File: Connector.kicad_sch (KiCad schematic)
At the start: 1 part, among them J6 2-338069-0

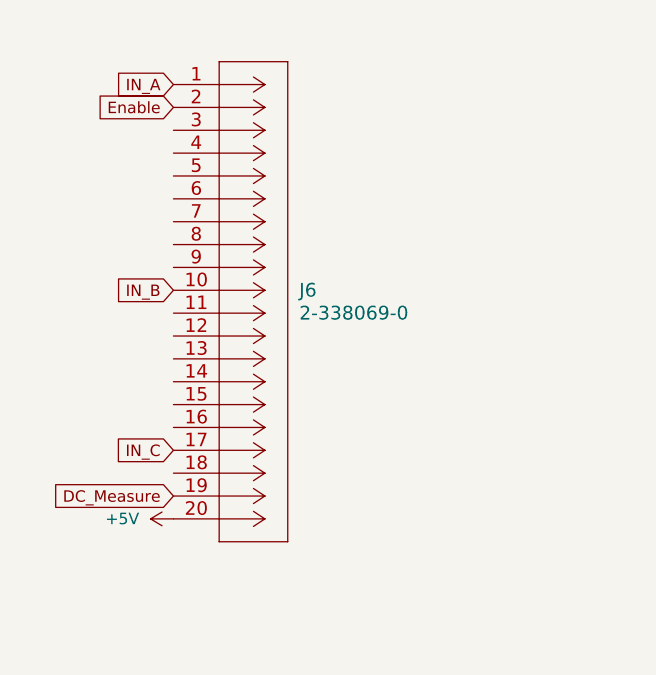
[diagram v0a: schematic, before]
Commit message: Стартовый вариант
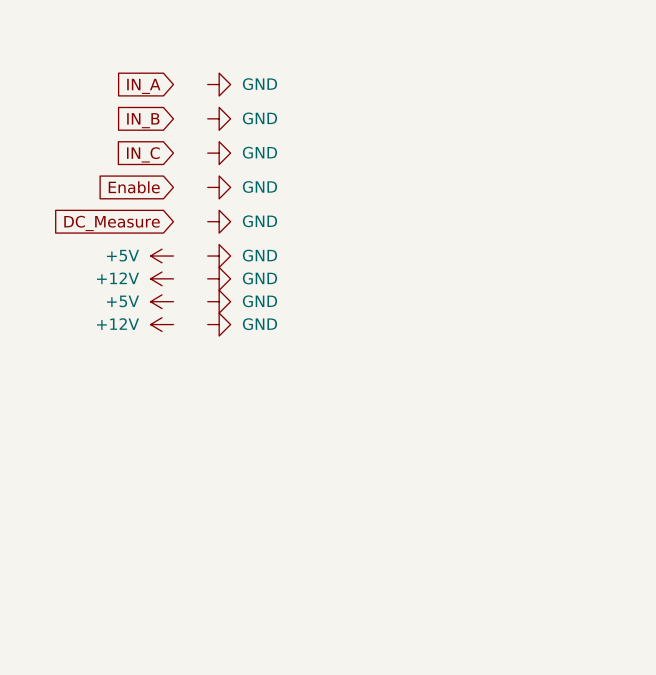
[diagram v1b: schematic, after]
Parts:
- removed J6: 2-338069-0, Connector_My:2-338069-0, symbol Connector_My:2-338069-0

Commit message: Стартовая версия
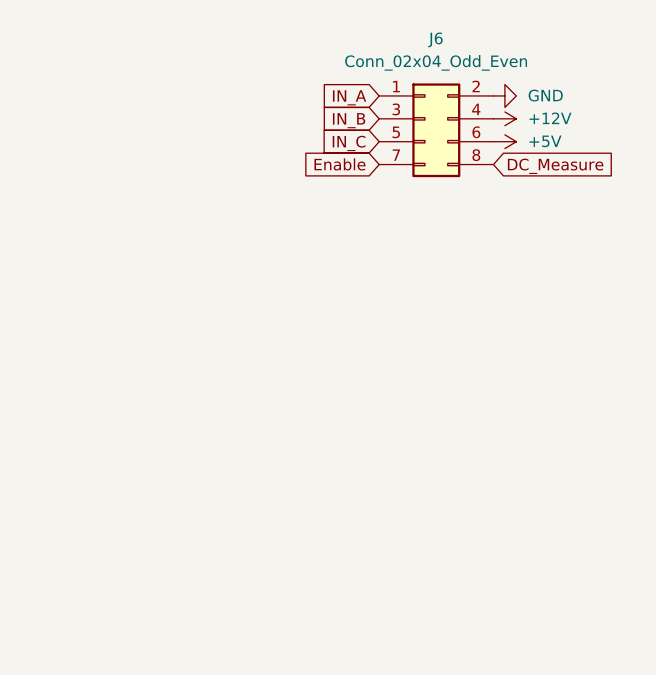
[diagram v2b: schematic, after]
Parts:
- added J6: Conn_02x04_Odd_Even, Connector_PinHeader_2.54mm:PinHeader_2x04_P2.54mm_Vertical, symbol Connector_Generic:Conn_02x04_Odd_Even
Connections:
- net +12V: now also J6.4 (Pin_4)
- net +5V: now also J6.6 (Pin_6)
- net DC_Measure: now also J6.8 (Pin_8)
- net Enable: now also J6.7 (Pin_7)
- net GND: now also J6.2 (Pin_2)
- net IN_A: now also J6.1 (Pin_1)
- net IN_B: now also J6.3 (Pin_3)
- net IN_C: now also J6.5 (Pin_5)

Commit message: Стартовая версия
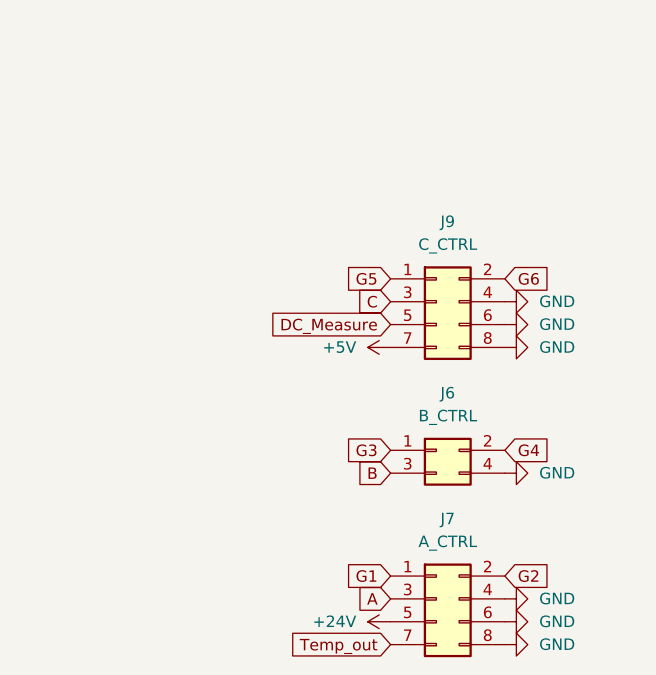
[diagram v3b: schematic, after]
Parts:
- removed J6: Conn_02x04_Odd_Even, Connector_PinHeader_2.54mm:PinHeader_2x04_P2.54mm_Vertical, symbol Connector_Generic:Conn_02x04_Odd_Even
- added J6: B_CTRL, Connector_PinSocket_2.54mm:PinSocket_2x02_P2.54mm_Vertical_SMD, symbol Connector_Generic:Conn_02x02_Odd_Even
- added J7: A_CTRL, Connector_PinSocket_2.54mm:PinSocket_2x04_P2.54mm_Vertical_SMD, symbol Connector_Generic:Conn_02x04_Odd_Even
- added J9: C_CTRL, Connector_PinSocket_2.54mm:PinSocket_2x04_P2.54mm_Vertical_SMD, symbol Connector_Generic:Conn_02x04_Odd_Even
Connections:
- net +5V: now also J9.7 (Pin_7)
- net DC_Measure: now also J9.5 (Pin_5)
- net GND: now also J6.4 (Pin_4), J7.4 (Pin_4), J7.6 (Pin_6), J7.8 (Pin_8), J9.4 (Pin_4), J9.6 (Pin_6), J9.8 (Pin_8)
- new net +24V: J7.5 (Pin_5)
- new net A: J7.3 (Pin_3)
- new net B: J6.3 (Pin_3)
- new net C: J9.3 (Pin_3)
- new net G1: J7.1 (Pin_1)
- new net G2: J7.2 (Pin_2)
- new net G3: J6.1 (Pin_1)
- new net G4: J6.2 (Pin_2)
- new net G5: J9.1 (Pin_1)
- new net G6: J9.2 (Pin_2)
- new net Temp_out: J7.7 (Pin_7)

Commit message: Стартовая версия
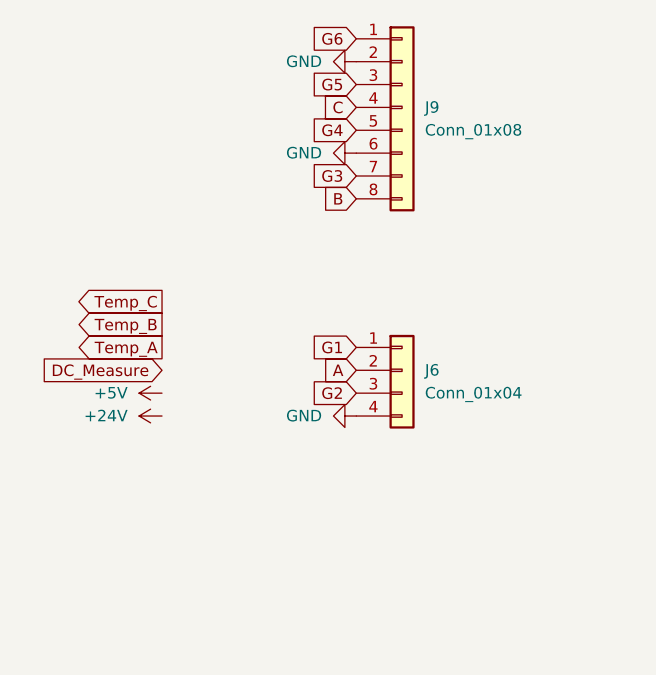
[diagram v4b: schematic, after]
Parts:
- removed J6: B_CTRL, Connector_PinSocket_2.54mm:PinSocket_2x02_P2.54mm_Vertical_SMD, symbol Connector_Generic:Conn_02x02_Odd_Even
- removed J7: A_CTRL, Connector_PinSocket_2.54mm:PinSocket_2x04_P2.54mm_Vertical_SMD, symbol Connector_Generic:Conn_02x04_Odd_Even
- removed J9: C_CTRL, Connector_PinSocket_2.54mm:PinSocket_2x04_P2.54mm_Vertical_SMD, symbol Connector_Generic:Conn_02x04_Odd_Even
- added J6: Conn_01x04, Connector_PinHeader_2.54mm:PinHeader_1x04_P2.54mm_Vertical, symbol Connector_Generic:Conn_01x04
- added J9: Conn_01x08, Connector_PinHeader_2.54mm:PinHeader_1x08_P2.54mm_Vertical, symbol Connector_Generic:Conn_01x08
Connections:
- net A: now also J6.2 (Pin_2)
- net B: now also J9.8 (Pin_8)
- net C: now also J9.4 (Pin_4)
- net G1: now also J6.1 (Pin_1)
- net G2: now also J6.3 (Pin_3)
- net G3: now also J9.7 (Pin_7)
- net G4: now also J9.5 (Pin_5)
- net G5: now also J9.3 (Pin_3)
- net G6: now also J9.1 (Pin_1)
- net GND: now also J6.4 (Pin_4), J9.2 (Pin_2), J9.6 (Pin_6)
